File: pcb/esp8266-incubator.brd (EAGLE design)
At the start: 48.3 x 91.7 mm, 48 parts, among them Q1 MOSFET-PGDS_TO220V

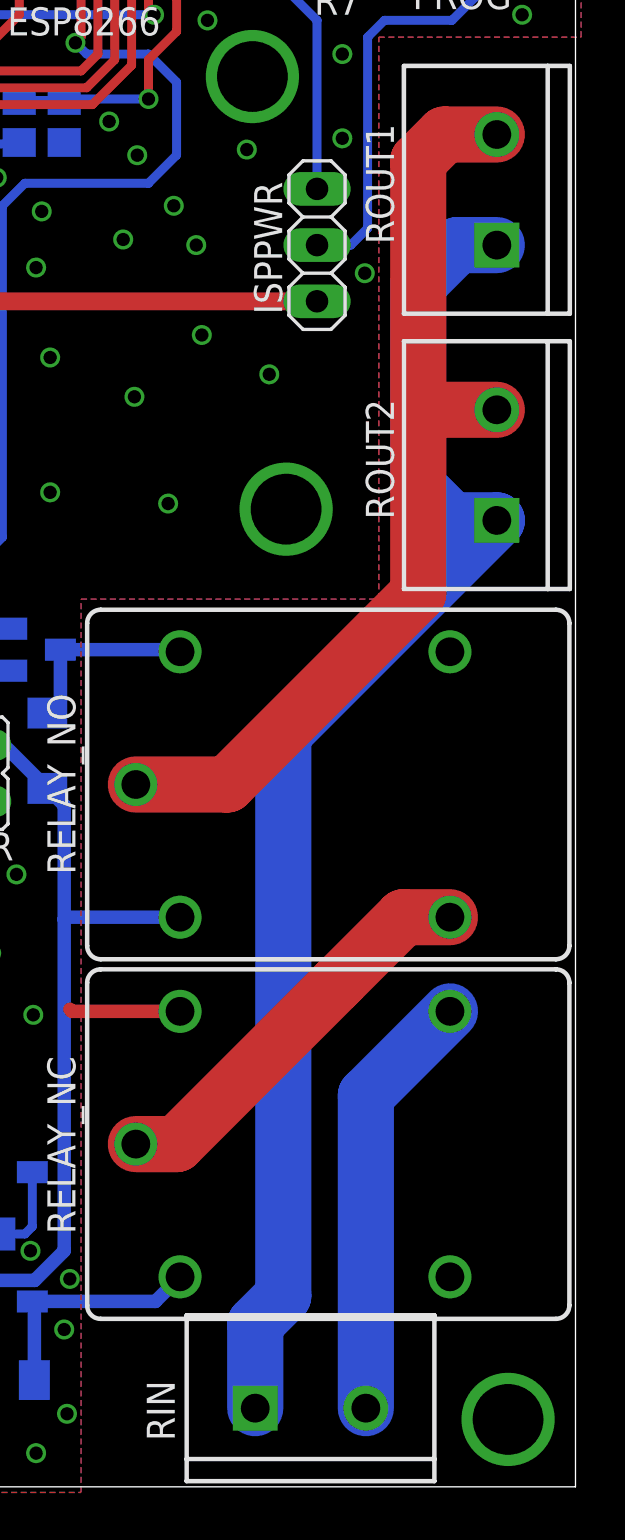
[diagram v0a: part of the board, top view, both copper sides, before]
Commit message: Renamed source files.
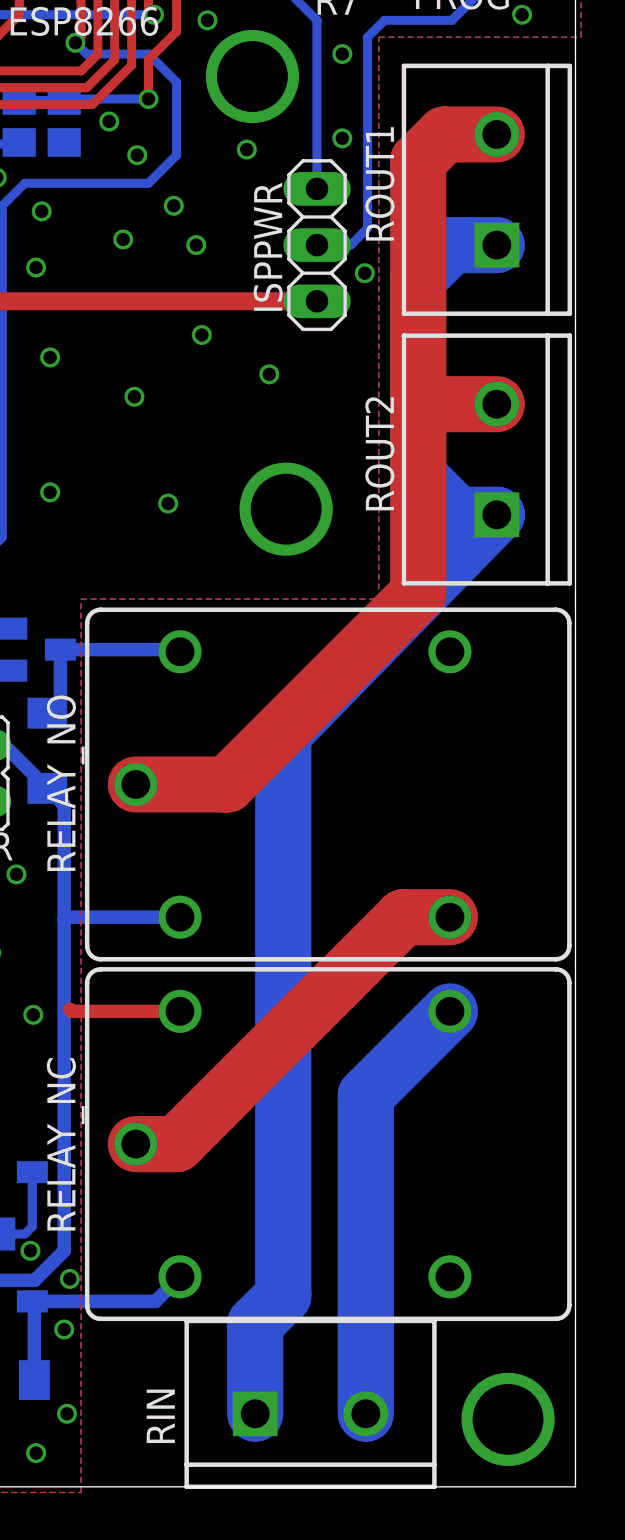
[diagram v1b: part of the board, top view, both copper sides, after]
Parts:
- C4: value 100nF -> 1000nF
- D3: value (none) -> 1N4007
- R12, R13, R14, R15: value 12K -> 10K
- R17: value 12K -> 100R
- R18: value 12K -> 120K
- moved RIN 0.25 mm to (33.8, 3.30)
- moved ROUT2 0.25 mm to (44.7, 43.9)
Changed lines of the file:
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@@
 <attribute name="VALUE" x="20.701" y="35.941" size="1.27" layer="28" rot="MR90"/>
 </element>
-<element name="RIN" library="SparkFun-Connectors" package="SCREWTERMINAL-5MM-2" value="" x="33.782" y="3.556" smashed="yes">
-<attribute name="NAME" x="30.146" y="2.08" size="1.27" layer="25" font="vector" ratio="15" rot="R90"/>
-<attribute name="STOREFRONT_ID" value="PRT-08432" x="33.782" y="3.556" size="1.778" layer="27" display="off"/>
+<element name="RIN" library="SparkFun-Connectors" package="SCREWTERMINAL-5MM-2" value="" x="33.782" y="3.302" smashed="yes">
+<attribute name="NAME" x="30.146" y="1.826" size="1.27" layer="25" font="vector" ratio="15" rot="R90"/>
+<attribute name="STOREFRONT_ID" value="PRT-08432" x="33.782" y="3.302" size="1.778" layer="27" display="off"/>
 </element>
 <element name="ROUT1" library="SparkFun-Connectors" package="SCREWTERMINAL-5MM-2" value="" x="44.704" y="56.134" smashed="yes" rot="R90">
@@
 <attribute name="VALUE" x="24.257" y="2.159" size="1.27" layer="28" ratio="10" rot="MR0"/>
 </element>
-<element name="R12" library="rcl" package="R0805" value="12K" x="19.304" y="14.732" smashed="yes" rot="MR90">
+<element name="R12" library="rcl" package="R0805" value="10K" x="19.304" y="14.732" smashed="yes" rot="MR90">
 <attribute name="NAME" x="18.288" y="16.637" size="1.27" layer="26" font="vector" ratio="15" rot="MR270"/>
 <attribute name="VALUE" x="16.764" y="14.097" size="1.27" layer="28" rot="MR90"/>
@@
 <attribute name="VALUE" x="19.431" y="12.319" size="1.27" layer="28" rot="MR90"/>
 </element>
-<element name="R13" library="rcl" package="R0805" value="12K" x="21.336" y="11.43" smashed="yes" rot="MR180">
+<element name="R13" library="rcl" package="R0805" value="10K" x="21.336" y="11.43" smashed="yes" rot="MR180">
 <attribute name="NAME" x="19.431" y="10.922" size="1.27" layer="26" font="vector" ratio="15" rot="MR0"/>
 <attribute name="VALUE" x="20.701" y="13.97" size="1.27" layer="28" rot="MR180"/>
 </element>
-<element name="R14" library="rcl" package="R0805" value="12K" x="20.066" y="36.83" smashed="yes" rot="MR0">
+<element name="R14" library="rcl" package="R0805" value="10K" x="20.066" y="36.83" smashed="yes" rot="MR0">
 <attribute name="NAME" x="14.351" y="37.338" size="1.27" layer="26" font="vector" ratio="15" rot="MR180"/>
 <attribute name="VALUE" x="20.701" y="34.29" size="1.27" layer="28" rot="MR0"/>
@@
 <attribute name="VALUE" x="19.431" y="6.477" size="1.27" layer="28" rot="MR90"/>
 </element>
-<element name="R15" library="rcl" package="R0805" value="12K" x="19.304" y="8.382" smashed="yes" rot="MR270">
+<element name="R15" library="rcl" package="R0805" value="10K" x="19.304" y="8.382" smashed="yes" rot="MR270">
 <attribute name="NAME" x="18.288" y="10.287" size="1.27" layer="26" font="vector" ratio="15" rot="MR270"/>
 <attribute name="VALUE" x="21.844" y="9.017" size="1.27" layer="28" rot="MR270"/>
 </element>
-<element name="ROUT2" library="SparkFun-Connectors" package="SCREWTERMINAL-5MM-2" value="" x="44.704" y="43.688" smashed="yes" rot="R90">
-<attribute name="NAME" x="40.052" y="43.736" size="1.27" layer="25" font="vector" ratio="15" rot="R90"/>
-<attribute name="STOREFRONT_ID" value="PRT-08432" x="44.704" y="43.688" size="1.778" layer="27" rot="R90" display="off"/>
+<element name="ROUT2" library="SparkFun-Connectors" package="SCREWTERMINAL-5MM-2" value="" x="44.704" y="43.942" smashed="yes" rot="R90">
+<attribute name="NAME" x="40.052" y="43.99" size="1.27" layer="25" font="vector" ratio="15" rot="R90"/>
+<attribute name="STOREFRONT_ID" value="PRT-08432" x="44.704" y="43.942" size="1.778" layer="27" rot="R90" display="off"/>
 </element>
 <element name="ALARM" library="SparkFun" package="BUZZER-12MM" value="BUZZERPTH" x="8.636" y="72.898" smashed="yes">
@@
 <attribute name="VALUE" x="14.478" y="63.246" size="1.27" layer="27" ratio="10" rot="R270"/>
 </element>
-<element name="R17" library="rcl" package="R0805" value="12K" x="23.114" y="61.722" smashed="yes" rot="MR90">
+<element name="R17" library="rcl" package="R0805" value="100R" x="23.114" y="61.722" smashed="yes" rot="MR90">
 <attribute name="NAME" x="23.876" y="59.563" size="1.27" layer="26" font="vector" ratio="15" rot="MR270"/>
 <attribute name="VALUE" x="20.574" y="61.087" size="1.27" layer="28" rot="MR90"/>
 </element>
-<element name="R18" library="rcl" package="R0805" value="12K" x="25.146" y="61.722" smashed="yes" rot="MR90">
+<element name="R18" library="rcl" package="R0805" value="120K" x="25.146" y="61.722" smashed="yes" rot="MR90">
 <attribute name="NAME" x="25.908" y="59.563" size="1.27" layer="26" font="vector" ratio="15" rot="MR270"/>
 <attribute name="VALUE" x="22.606" y="61.087" size="1.27" layer="28" rot="MR90"/>
 </element>
-<element name="D3" library="diode" package="MELF-MLL41" value="" x="9.398" y="43.688" smashed="yes" rot="MR90">
+<element name="D3" library="diode" package="MELF-MLL41" value="1N4007" x="9.398" y="43.688" smashed="yes" rot="MR90">
 <attribute name="NAME" x="11.303" y="42.672" size="1.27" layer="26" font="vector" ratio="15" rot="MR90"/>
 <attribute name="VALUE" x="7.112" y="41.148" size="0.4064" layer="28" font="vector" rot="MR90"/>
 </element>
-<element name="C4" library="rcl" package="C0805" value="100nF" x="6.604" y="43.688" smashed="yes" rot="MR270">
+<element name="C4" library="rcl" package="C0805" value="1000nF" x="6.604" y="43.688" smashed="yes" rot="MR270">
 <attribute name="NAME" x="7.112" y="41.656" size="1.27" layer="26" font="vector" ratio="15" rot="MR270"/>
 <attribute name="VALUE" x="9.144" y="44.958" size="1.27" layer="28" rot="MR270"/>
@@
 <wire x1="44.704" y1="61.134" x2="42.338" y2="61.134" width="2.54" layer="1"/>
 <wire x1="42.338" y1="61.134" x2="41.148" y2="59.944" width="2.54" layer="1"/>
-<wire x1="41.148" y1="59.944" x2="41.148" y2="48.514" width="2.54" layer="1"/>
-<wire x1="41.148" y1="48.514" x2="41.148" y2="40.386" width="2.54" layer="1"/>
+<wire x1="41.148" y1="59.944" x2="41.148" y2="49.022" width="2.54" layer="1"/>
+<wire x1="41.148" y1="48.942" x2="41.148" y2="40.386" width="2.54" layer="1"/>
 <wire x1="41.148" y1="40.386" x2="32.512" y2="31.75" width="2.54" layer="1"/>
 <wire x1="32.512" y1="31.75" x2="28.384" y2="31.75" width="2.54" layer="1"/>
-<wire x1="44.704" y1="48.688" x2="41.322" y2="48.688" width="2.54" layer="1"/>
-<wire x1="41.322" y1="48.688" x2="41.148" y2="48.514" width="2.54" layer="1"/>
+<wire x1="44.704" y1="48.942" x2="41.148" y2="48.942" width="2.54" layer="1"/>
+<wire x1="41.148" y1="48.942" x2="41.148" y2="49.022" width="2.54" layer="1"/>
 </signal>
 <signal name="N$17">
@@
 <contactref element="ROUT1" pad="1"/>
 <contactref element="ROUT2" pad="1"/>
-<wire x1="33.782" y1="3.556" x2="33.782" y2="7.366" width="2.54" layer="16"/>
+<wire x1="33.782" y1="3.302" x2="33.782" y2="7.366" width="2.54" layer="16"/>
 <wire x1="33.782" y1="7.366" x2="35.052" y2="8.636" width="2.54" layer="16"/>
 <wire x1="35.052" y1="8.636" x2="35.052" y2="34.036" width="2.54" layer="16"/>
-<wire x1="35.052" y1="34.036" x2="44.704" y2="43.688" width="2.54" layer="16"/>
-<wire x1="44.704" y1="43.688" x2="42.672" y2="43.688" width="2.54" layer="16"/>
-<wire x1="42.672" y1="43.688" x2="41.148" y2="45.212" width="2.54" layer="16"/>
-<wire x1="44.704" y1="56.134" x2="42.926" y2="56.134" width="2.54" layer="16"/>
-<wire x1="42.926" y1="56.134" x2="41.148" y2="54.356" width="2.54" layer="16"/>
-<wire x1="41.148" y1="54.356" x2="41.148" y2="45.212" width="2.54" layer="16"/>
+<wire x1="35.052" y1="34.036" x2="44.704" y2="43.942" width="2.54" layer="16"/>
+<wire x1="44.704" y1="43.942" x2="42.926" y2="43.942" width="2.54" layer="16"/>
+<wire x1="42.926" y1="43.942" x2="41.148" y2="45.72" width="2.54" layer="16"/>
+<wire x1="41.148" y1="45.72" x2="41.148" y2="54.61" width="2.54" layer="16"/>
+<wire x1="44.704" y1="56.134" x2="42.672" y2="56.134" width="2.54" layer="16"/>
+<wire x1="42.672" y1="56.134" x2="41.148" y2="54.61" width="2.54" layer="16"/>
 </signal>
 <signal name="P230">
 <contactref element="RELAY_NC" pad="NC"/>
 <contactref element="RIN" pad="2"/>
-<wire x1="38.782" y1="3.556" x2="38.782" y2="17.692" width="2.54" layer="16"/>
+<wire x1="38.782" y1="3.302" x2="38.782" y2="17.692" width="2.54" layer="16"/>
 <wire x1="38.782" y1="17.692" x2="42.584" y2="21.494" width="2.54" layer="16"/>
 </signal>
